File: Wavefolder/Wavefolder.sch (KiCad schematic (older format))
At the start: 58 parts, among them J1 EuroPower, J2 Sig1, J3 Out1, J4 Sig2, J5 CV2, J6 Out2, Q1 BC557, Q2 BC547, Q3 BC557, Q4 BC547, Q5 BC557, Q6 BC547, U1 TL074, U2 TL082, U3 TL082, U4 TL074

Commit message: Wavefolder done !
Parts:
- U2, U3: footprint Package_DIP:DIP-8_W7.62mm_LongPads -> Package_SO:SOIC-8_3.9x4.9mm_P1.27mm
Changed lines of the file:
@@
 F 0 "U2" H 4908 1196 50  0000 L CNN
 F 1 "TL082" H 4908 1105 50  0000 L CNN
-F 2 "Package_DIP:DIP-8_W7.62mm_LongPads" H 4950 1150 50  0001 C CNN
+F 2 "Package_SO:SOIC-8_3.9x4.9mm_P1.27mm" H 4950 1150 50  0001 C CNN
 F 3 "http://www.ti.com/lit/ds/symlink/tl081.pdf" H 4950 1150 50  0001 C CNN
 	3    4950 1150
@@
 F 0 "U3" H 5758 1196 50  0000 L CNN
 F 1 "TL082" H 5758 1105 50  0000 L CNN
-F 2 "Package_DIP:DIP-8_W7.62mm_LongPads" H 5800 1150 50  0001 C CNN
+F 2 "Package_SO:SOIC-8_3.9x4.9mm_P1.27mm" H 5800 1150 50  0001 C CNN
 F 3 "http://www.ti.com/lit/ds/symlink/tl081.pdf" H 5800 1150 50  0001 C CNN
 	3    5800 1150

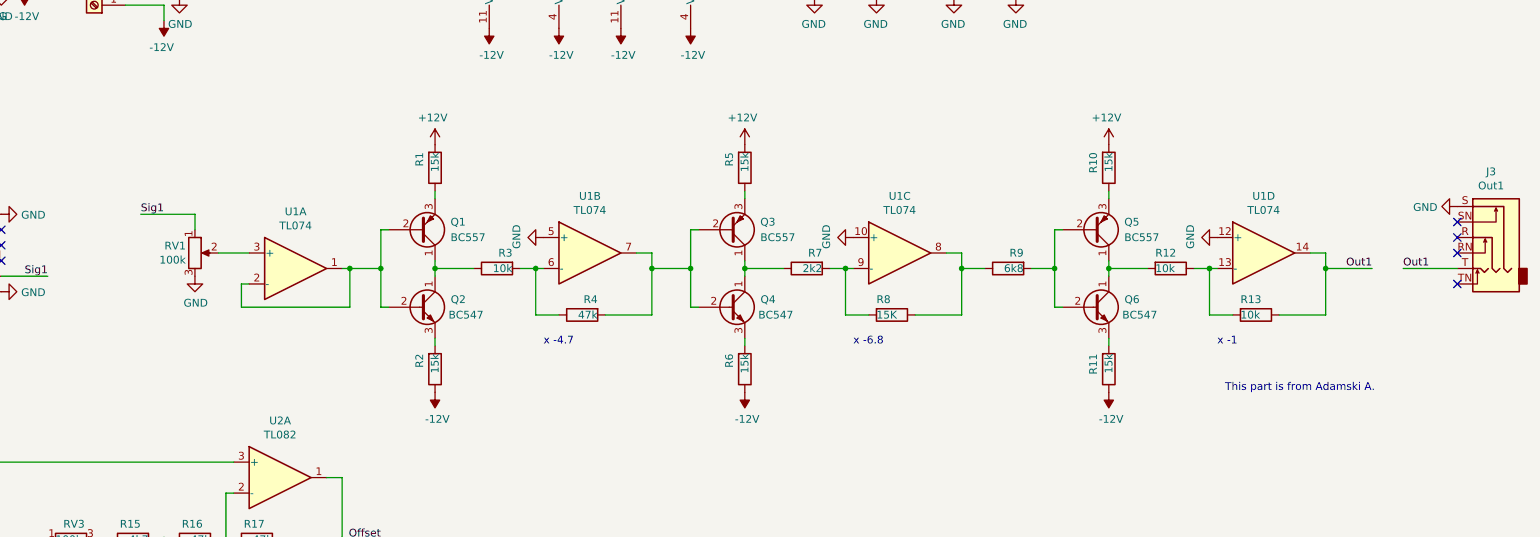
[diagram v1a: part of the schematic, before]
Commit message: Wavefolder done and tested!
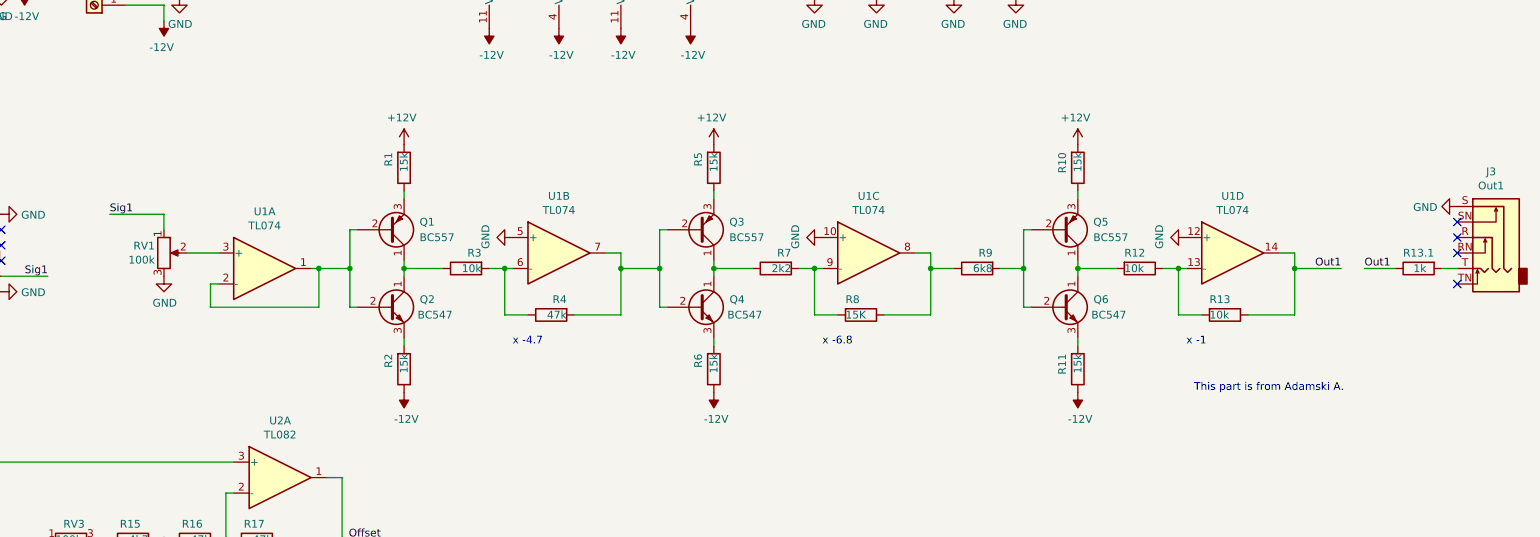
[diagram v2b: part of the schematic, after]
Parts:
- added R13.1: 1k, Resistor_THT:R_Axial_DIN0204_L3.6mm_D1.6mm_P2.54mm_Vertical, symbol Device:R
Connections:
- net Out1: now also R13.1.1; no longer J3.T
- new net: J3.T, R13.1.2
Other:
- moved on the sheet: Q1, Q2, Q3, Q4, Q5, Q6, R1, R10, R11, R12, R13, R2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
